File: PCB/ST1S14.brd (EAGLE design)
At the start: 97 x 50 mm, 16 parts

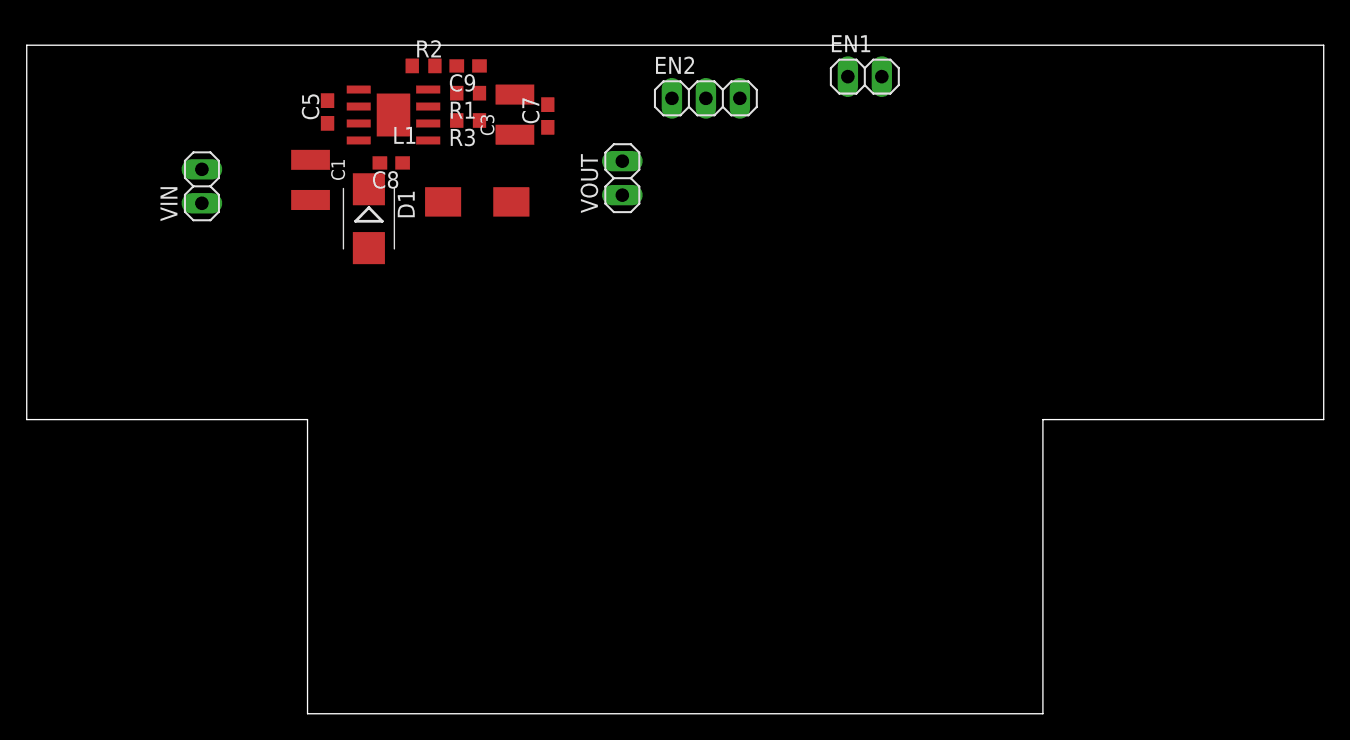
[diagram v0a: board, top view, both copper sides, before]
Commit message: Some changes on PCB
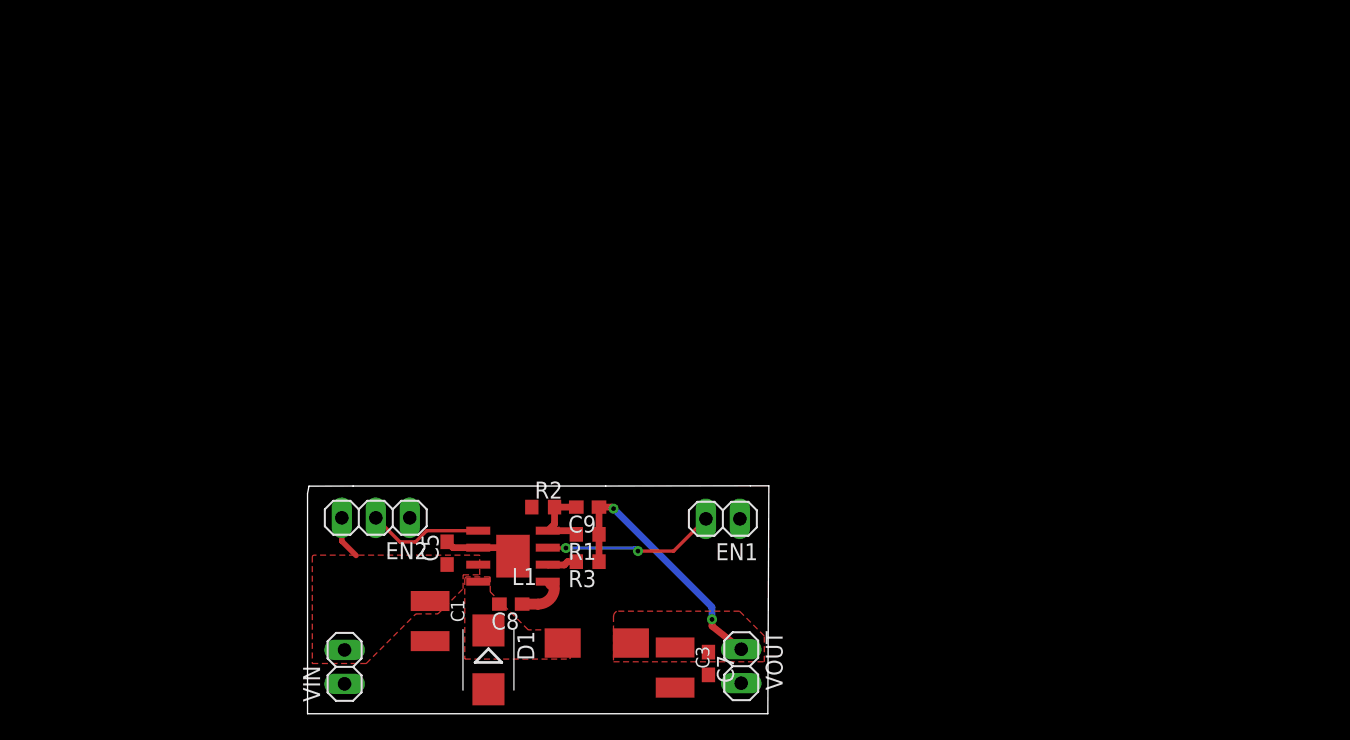
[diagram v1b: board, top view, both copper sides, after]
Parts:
- moved C3 43.0 mm to (27.5, 3.46), turned to 270 degrees
- moved C7 42.7 mm to (30.0, 3.76), turned to 270 degrees
- moved EN2 39.9 mm to (5.11, 14.7), turned to 180 degrees
- moved VOUT 37.6 mm to (32.4, 3.56), turned to 270 degrees
- moved VIN 37.5 mm to (2.77, 3.51)
- moved EN1 34.7 mm to (31.1, 14.6), turned to 180 degrees
- moved C5 34.2 mm to (10.4, 12.0)
- moved C9 34.2 mm to (21.0, 15.5)
- moved R2 34.2 mm to (17.6, 15.5)
- moved C1 34.2 mm to (9.17, 6.93)
- moved C8 34.2 mm to (15.2, 8.20)
- moved D1 34.2 mm to (13.5, 4.03)
- moved L1 34.2 mm to (21.1, 5.29)
- moved R1 34.2 mm to (21.0, 13.4)
- moved R3 34.2 mm to (21.0, 11.4)
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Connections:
- removed net N$5: C1.1, C5.1, U$1.7, VIN.2
- net VIN: now also C1.1, C5.1, U$1.7, VIN.2
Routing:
- net VOUT: track 0.00 -> 19.8 mm, vias 0 -> 2
- net EN1: track 0.00 -> 12.9 mm, vias 0 -> 2
- net EN2: track 0.00 -> 8.76 mm
- net N$2: track 0.00 -> 5.85 mm
- net GND: track 0.00 -> 4.52 mm
- net N$1: track 0.00 -> 3.61 mm
- net VIN: track 0.00 -> 3.26 mm
- net N$7: track 0.00 -> 2.25 mm
- added copper zone on layer 1, net N$3
- added copper zone on layer 1, net VIN
- added copper zone on layer 1, net VOUT
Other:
- board size 97 x 50 mm -> 34.5 x 17 mm
